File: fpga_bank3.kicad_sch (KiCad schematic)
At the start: 1 part, among them U2 XC7A50T-FGG484

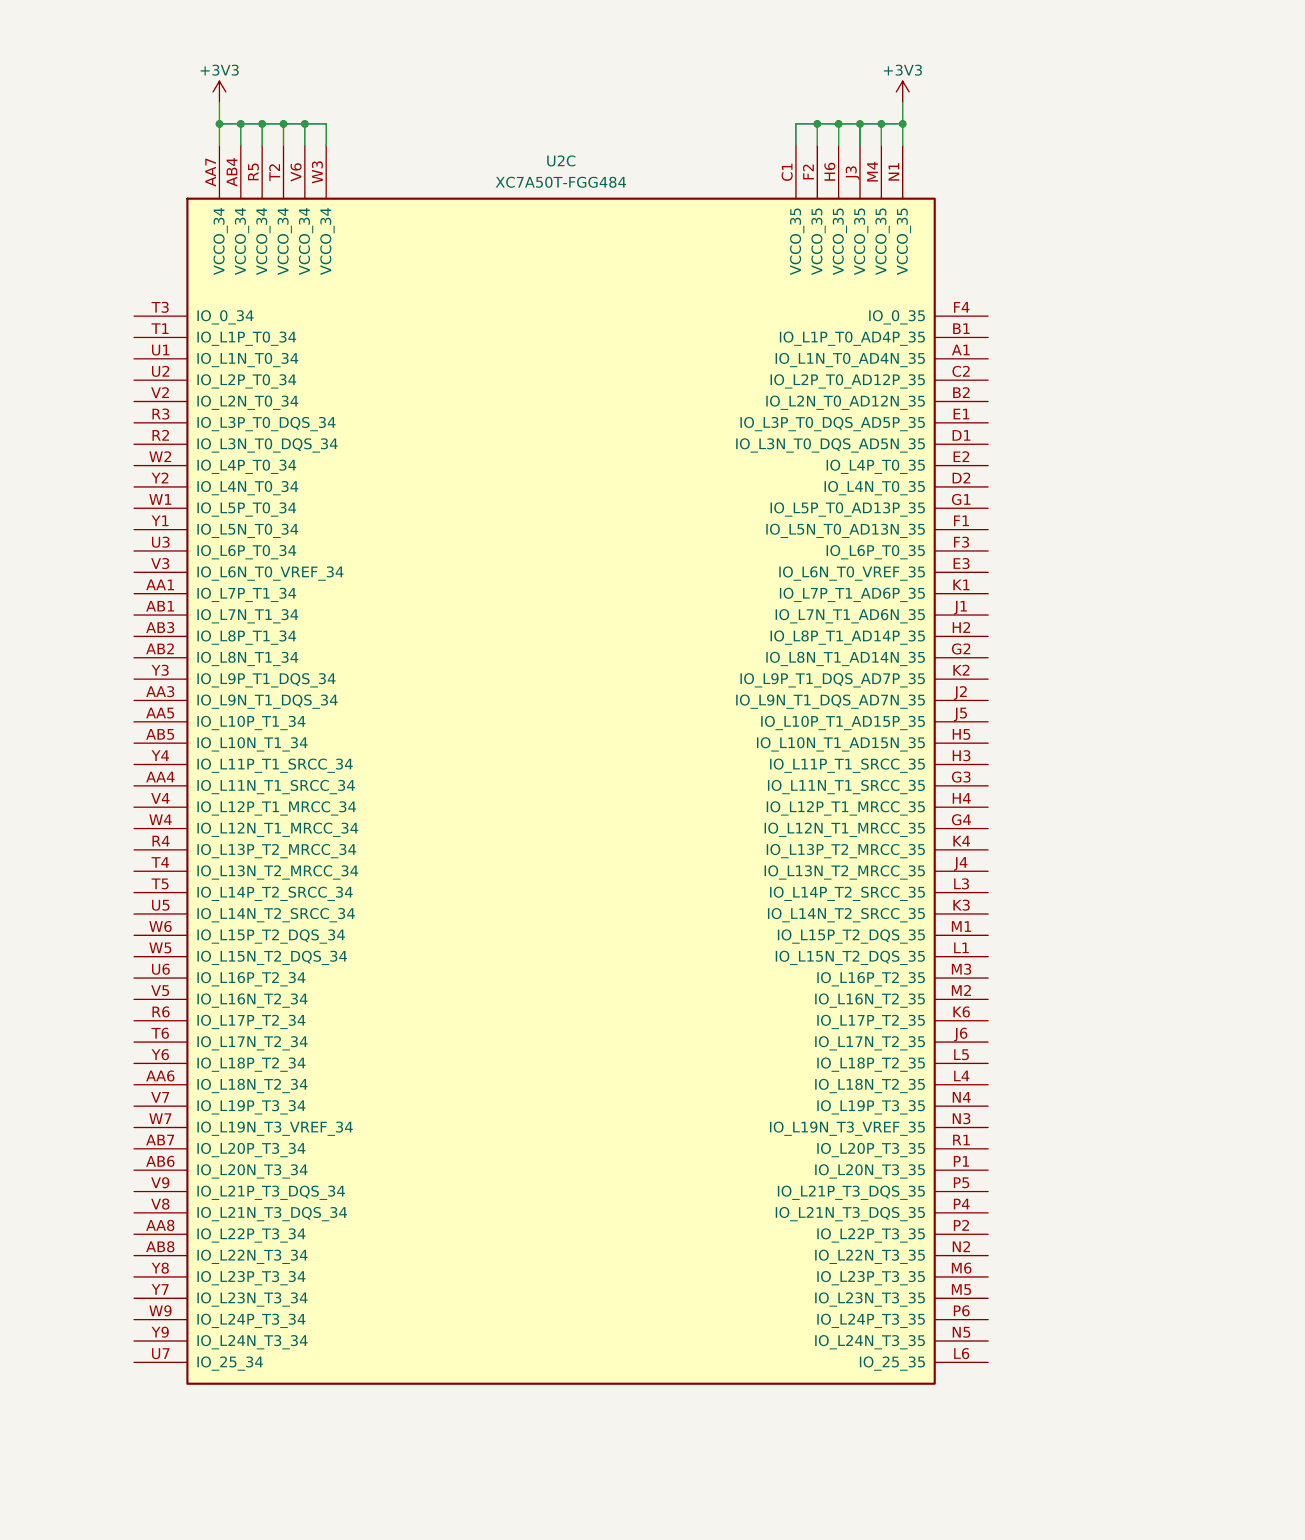
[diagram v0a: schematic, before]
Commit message: Schematic finished, starting layout
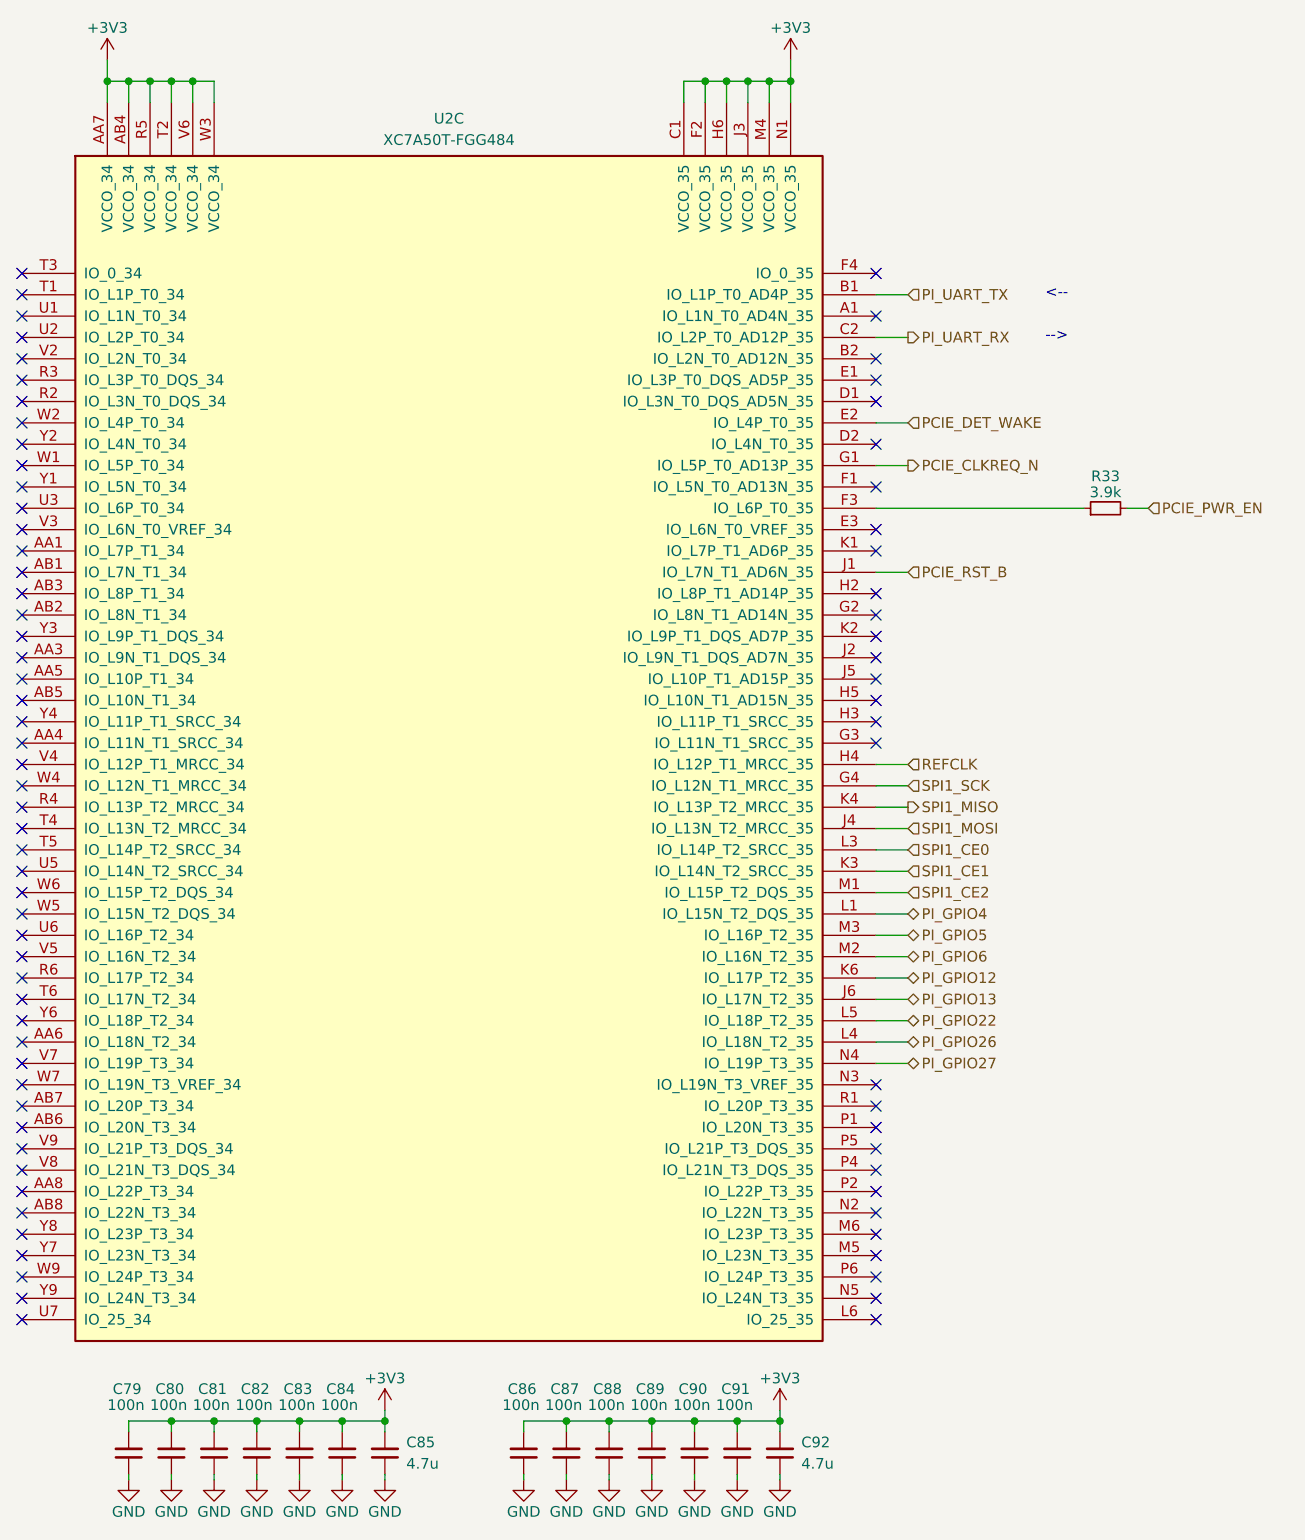
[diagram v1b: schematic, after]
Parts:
- added C79, C80, C81, C82, C83, C84, C86, C87, C88, C89, C90, C91: 100n, Capacitor_SMD:C_0402_1005Metric_Pad0.74x0.62mm_HandSolder, symbol Device:C_Small
- added C85, C92: 4.7u, Capacitor_SMD:C_0402_1005Metric_Pad0.74x0.62mm_HandSolder, symbol Device:C_Small
- added R33: 3.9k, Resistor_SMD:R_0402_1005Metric_Pad0.72x0.64mm_HandSolder, symbol Device:R_Small
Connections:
- net +3V3: now also C79.2, C80.2, C81.2, C82.2, C83.2, C84.2, C85.2, C86.2, C87.2, C88.2, C89.2, C90.2, C91.2, C92.2
- net PI_UART_TX: now reaches U2.B1 (IO_L1P_T0_AD4P_35)
- net PI_UART_RX: now reaches U2.C2 (IO_L2P_T0_AD12P_35)
- net PCIE_DET_WAKE: now reaches U2.E2 (IO_L4P_T0_35)
- net at U2.F3 (IO_L6P_T0_35): now also R33.1
- net PCIE_CLKREQ_N: now reaches U2.G1 (IO_L5P_T0_AD13P_35)
- net SPI1_SCK: now reaches U2.G4 (IO_L12N_T1_MRCC_35)
- net REFCLK: now reaches U2.H4 (IO_L12P_T1_MRCC_35)
- net PCIE_RST_B: now reaches U2.J1 (IO_L7N_T1_AD6N_35)
- net SPI1_MOSI: now reaches U2.J4 (IO_L13N_T2_MRCC_35)
- net PI_GPIO13: now reaches U2.J6 (IO_L17N_T2_35)
- net SPI1_CE1: now reaches U2.K3 (IO_L14N_T2_SRCC_35)
- net SPI1_MISO: now reaches U2.K4 (IO_L13P_T2_MRCC_35)
- net PI_GPIO12: now reaches U2.K6 (IO_L17P_T2_35)
- net PI_GPIO4: now reaches U2.L1 (IO_L15N_T2_DQS_35)
- net SPI1_CE0: now reaches U2.L3 (IO_L14P_T2_SRCC_35)
- net PI_GPIO26: now reaches U2.L4 (IO_L18N_T2_35)
- net PI_GPIO22: now reaches U2.L5 (IO_L18P_T2_35)
- net SPI1_CE2: now reaches U2.M1 (IO_L15P_T2_DQS_35)
- net PI_GPIO6: now reaches U2.M2 (IO_L16N_T2_35)
- net PI_GPIO5: now reaches U2.M3 (IO_L16P_T2_35)
- net PI_GPIO27: now reaches U2.N4 (IO_L19P_T3_35)
- new net GND: C79.1, C80.1, C81.1, C82.1, C83.1, C84.1, C85.1, C86.1, C87.1, C88.1, C89.1, C90.1, C91.1, C92.1
- new net PCIE_PWR_EN: R33.2
- no-connect marks 0 -> 79
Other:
- note added: "-->"
- note added: "<--"
- title: FPGA Bank 34 & 35 -> FPGA Power
- moved on the sheet: U2C
